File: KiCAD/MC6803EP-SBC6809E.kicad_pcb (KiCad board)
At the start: 2 copper layers, 57 x 60 mm, 5 parts, among them U1 MC6809E ソケット, U2 74HCT02, U3 MC6800

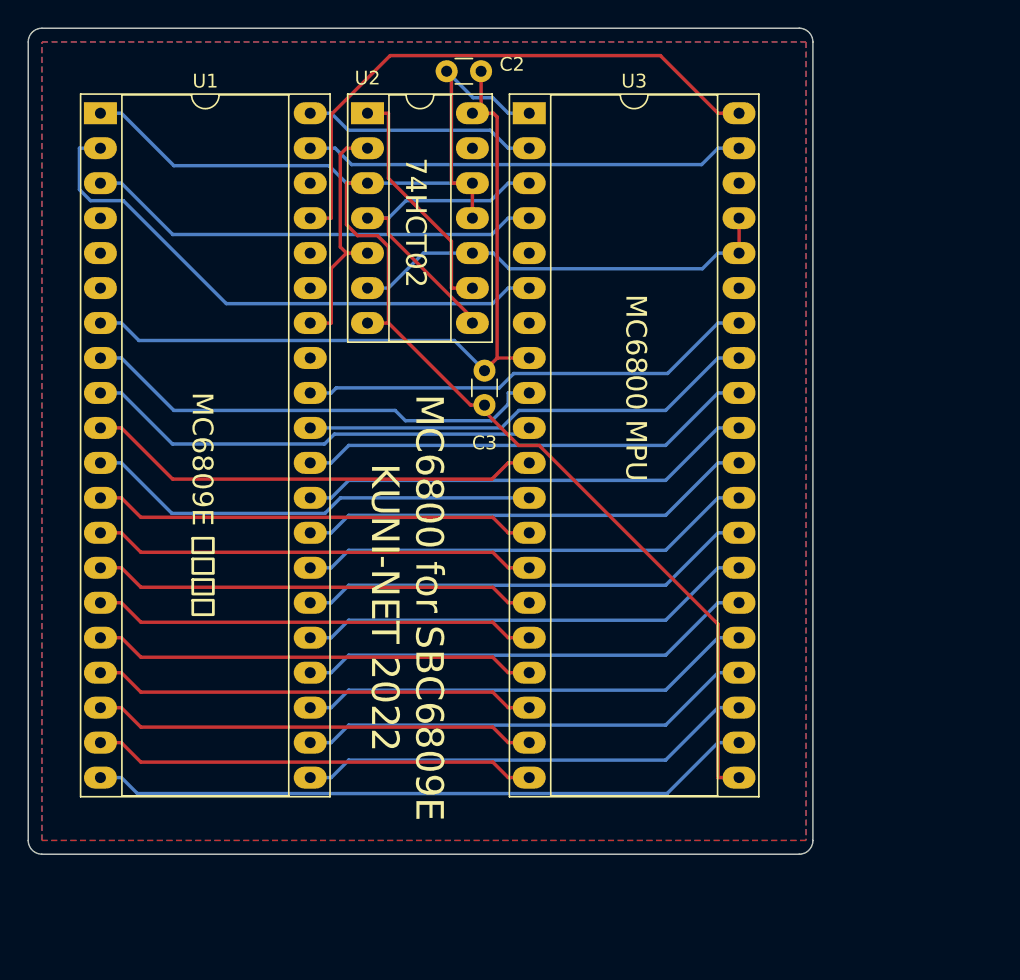
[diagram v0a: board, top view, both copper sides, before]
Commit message: REV1 ガーバーデータ出力
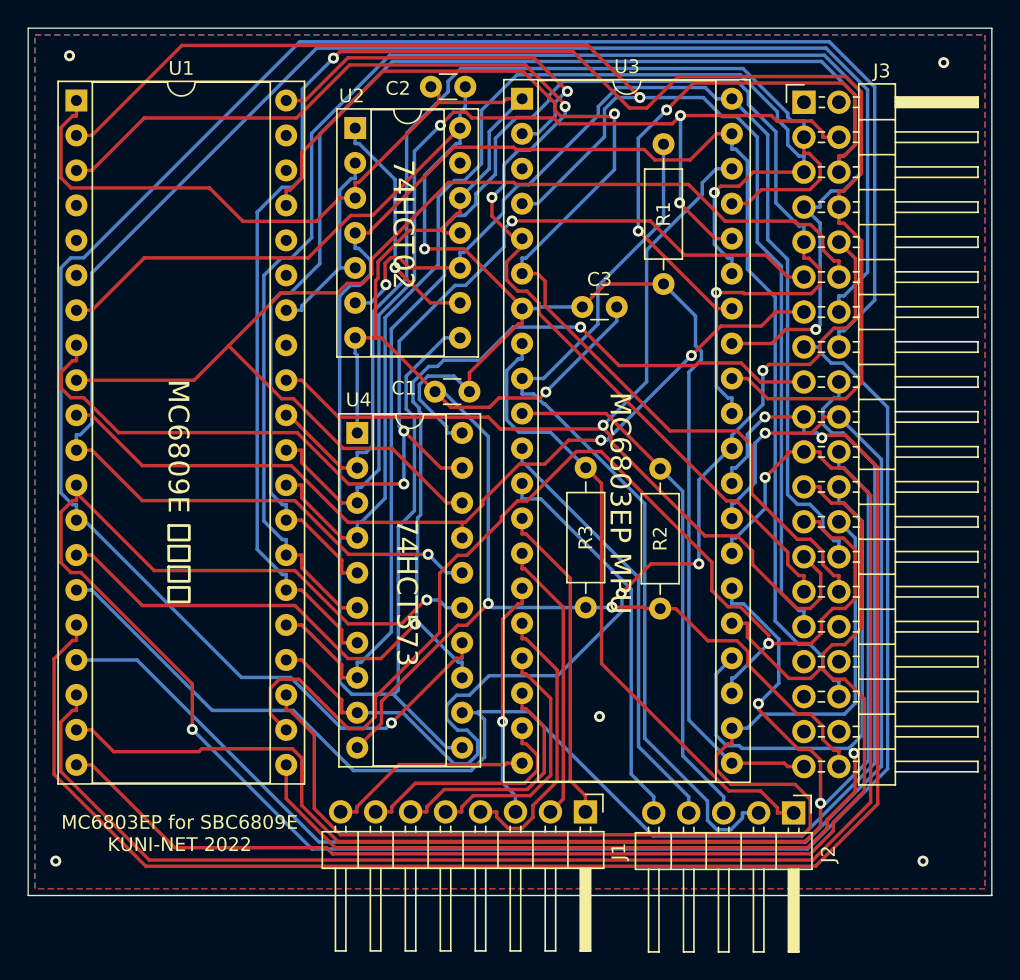
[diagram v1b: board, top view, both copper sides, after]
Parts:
- added C1: 0.1u, Capacitor_THT:C_Disc_D3.0mm_W1.6mm_P2.50mm, F.Cu at (138.1, 94.4)
- added J1: I/O PIN, Connector_PinHeader_2.54mm:PinHeader_1x08_P2.54mm_Horizontal, F.Cu at (146.5, 124.9)
- added J2: CONT PIN, Connector_PinHeader_2.54mm:PinHeader_1x05_P2.54mm_Horizontal, F.Cu at (161.6, 125.0)
- added J3: SBC68_BUS, Connector_PinHeader_2.54mm:PinHeader_2x20_P2.54mm_Horizontal, F.Cu at (162.3, 73.4)
- added R1: 10k, Resistor_THT:R_Axial_DIN0207_L6.3mm_D2.5mm_P10.16mm_Horizontal, F.Cu at (152.2, 86.6)
- added R2: 10k, Resistor_THT:R_Axial_DIN0207_L6.3mm_D2.5mm_P10.16mm_Horizontal, F.Cu at (151.9, 100.0)
- added R3: 10k, Resistor_THT:R_Axial_DIN0207_L6.3mm_D2.5mm_P10.16mm_Horizontal, F.Cu at (146.5, 99.9)
- added U4: 74LS573, Package_DIP:DIP-20_W7.62mm_Socket, F.Cu at (129.9, 97.4)
- U1: footprint Package_DIP:DIP-40_W15.24mm_Socket_LongPads -> Package_DIP:DIP-40_W15.24mm_Socket
- U2: footprint Package_DIP:DIP-14_W7.62mm_Socket_LongPads -> Package_DIP:DIP-14_W7.62mm_Socket
- U3: value MC6800 -> MC6803EP; footprint Package_DIP:DIP-40_W15.24mm_Socket_LongPads -> Package_DIP:DIP-40_W15.24mm_Socket
- moved C3 8.48 mm to (146.2, 88.2), turned to 0 degrees
- moved U1 1.98 mm to (109.5, 73.2)
- moved C2 1.61 mm to (137.8, 72.2)
- moved U2 1.40 mm to (129.8, 75.2)
- moved U3 1.17 mm to (141.9, 73.1)
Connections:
- U3 pad 10: /A1 -> Net-(J2-Pad3)
- U3 pad 11: /A2 -> Net-(J2-Pad4)
- U3 pad 12: /A3 -> Net-(J2-Pad5)
- U3 pad 13: /A4 -> Net-(J1-Pad1)
- U3 pad 14: /A5 -> Net-(J1-Pad2)
- U3 pad 15: /A6 -> Net-(J1-Pad3)
- U3 pad 16: /A7 -> Net-(J1-Pad4)
- U3 pad 17: /A8 -> Net-(J1-Pad5)
- U3 pad 18: /A9 -> Net-(J1-Pad6)
- U3 pad 19: /A10 -> Net-(J1-Pad7)
- U3 pad 20: /A11 -> Net-(J1-Pad8)
- U3 pad 21: GND -> VCC
- U3 pad 22: /A12 -> /A15
- U3 pad 23: /A13 -> /A14
- U3 pad 24: /A14 -> /A13
- U3 pad 25: /A15 -> /A12
- U3 pad 26: /D7 -> /A11
- U3 pad 27: /D6 -> /A10
- U3 pad 28: /D5 -> /A9
- U3 pad 29: /D4 -> /A8
- U3 pad 3: /PHI1 -> unconnected-(U3-Pad3)
- U3 pad 30: /D3 -> /D7
- U3 pad 31: /D2 -> /D6
- U3 pad 32: /D1 -> /D5
- U3 pad 33: /D0 -> /D4
- U3 pad 34: /R/~{W} -> /D3
- U3 pad 35: unconnected-(U3-Pad35) -> /D2
- U3 pad 36: /PHI2 -> /D1
- U3 pad 37: /PHI2 -> /D0
- U3 pad 38: unconnected-(U3-Pad38) -> /R/~{W}
- U3 pad 39: /TSC -> /PHI1
- U3 pad 4: /~{IRQ} -> /~{NMI}
- U3 pad 40: /~{RES} -> /PHI2
- U3 pad 5: unconnected-(U3-Pad5) -> /~{IRQ}
- U3 pad 6: /~{NMI} -> /~{RES}
- U3 pad 7: unconnected-(U3-Pad7) -> VCC
- U3 pad 8: VCC -> Net-(J2-Pad1)
- U3 pad 9: /A0 -> Net-(J2-Pad2)
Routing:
- net /PHI1: track 24.6 -> 150.7 mm
- net /A4: track 32.2 -> 146.6 mm, vias 0 -> 2
- net /A5: track 32.2 -> 144.1 mm, vias 0 -> 1
- net /A3: track 33.1 -> 126.8 mm, vias 0 -> 1
- net /D3: track 33.3 -> 126.2 mm, vias 0 -> 2
- net /D5: track 33.3 -> 124.8 mm, vias 0 -> 1
- net /A8: track 32.2 -> 117.2 mm, vias 0 -> 2
- net /A11: track 32.2 -> 110.5 mm, vias 0 -> 2
- net /D4: track 33.3 -> 111.3 mm, vias 0 -> 1
- net /A10: track 32.2 -> 108.5 mm, vias 0 -> 1
- net /A9: track 32.2 -> 106.3 mm, vias 0 -> 1
- net /A7: track 32.2 -> 105.3 mm
- net /D6: track 33.3 -> 105.6 mm, vias 0 -> 1
- net VCC: track 55.4 -> 127.0 mm, vias 0 -> 1
- net Net-(J2-Pad2): track 0.00 -> 65.1 mm
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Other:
- board size 57 x 60 mm -> 70 x 63 mm
- board text added: "10"
- board text added: "11"
- board text added: "12"
- board text added: "13"
- board text added: "14"
- board text added: "15"
- board text added: "16"
- board text added: "17"
- board text added: "20"
- board text added: "21"
- board text added: "22"
- board text added: "23"
- board text added: "24"
- board text added: "74HCT573"
- board text added: "MC6803EP MPU"
- board text added: "MC6803EP for SBC6809E KUNI-NET 2022"
- board text removed: "MC6800 MPU"
- board text removed: "MC6800 for SBC6809E KUNI-NET 2022"
